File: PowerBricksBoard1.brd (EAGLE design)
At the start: 76.2 x 50.8 mm, 16 parts

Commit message: trim
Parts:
- R5: value 475k -> 510k
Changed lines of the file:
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@@
 <attribute name="VALUE" x="58.0644" y="26.3398" size="0.6096" layer="27" font="vector" ratio="20" rot="R270" align="top-center"/>
 </element>
-<element name="R5" library="SparkFun-Resistors" library_urn="urn:adsk.eagle:library:532" package="0603" package3d_urn="urn:adsk.eagle:package:39650/1" value="475k" x="60.96" y="22.733" smashed="yes" rot="R270">
+<element name="R5" library="SparkFun-Resistors" library_urn="urn:adsk.eagle:library:532" package="0603" package3d_urn="urn:adsk.eagle:package:39650/1" value="510k" x="60.96" y="22.733" smashed="yes" rot="R270">
 <attribute name="NAME" x="61.721996875" y="22.733003125" size="0.6096" layer="25" font="vector" ratio="20" rot="R270" align="bottom-center"/>
 <attribute name="PROD_ID" value=" " x="-30.479996875" y="-64.896996875" size="1.778" layer="27" rot="R270" display="off"/>

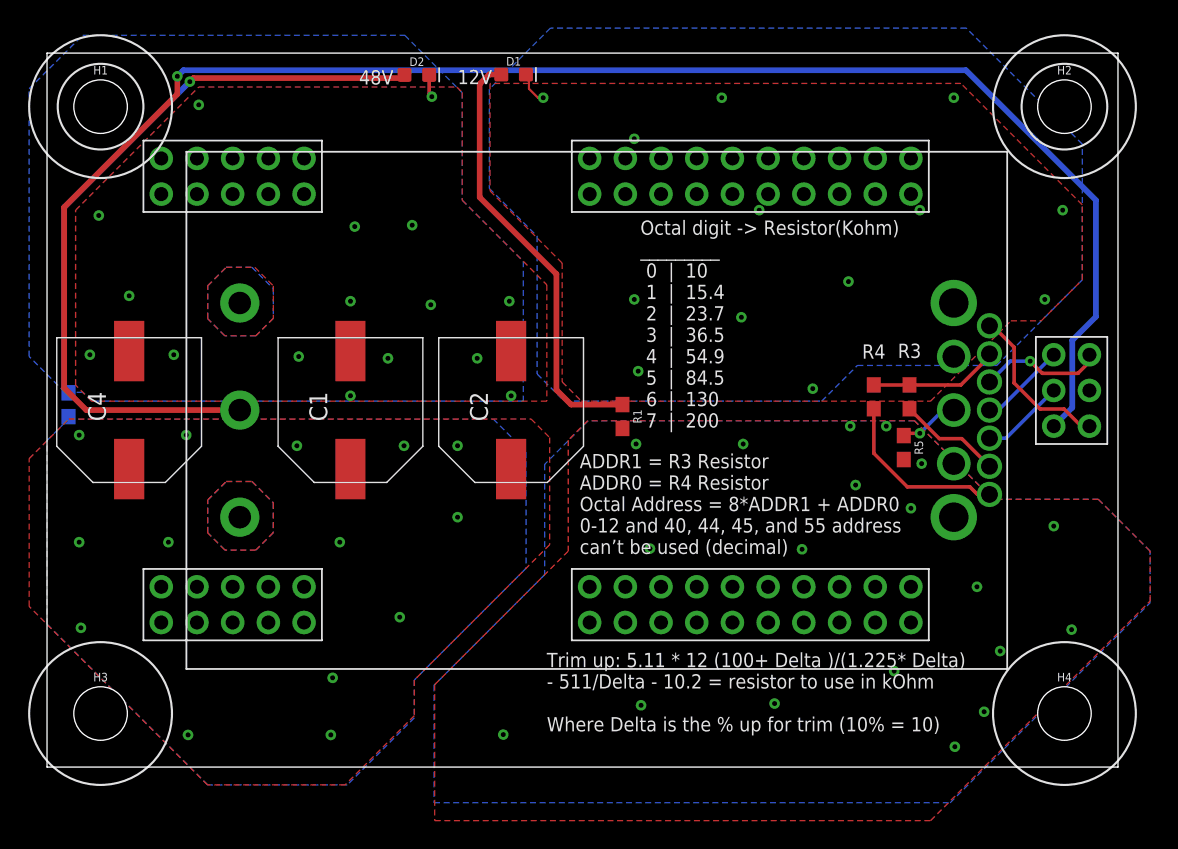
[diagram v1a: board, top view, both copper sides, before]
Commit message: Cleaning up git and exports for order
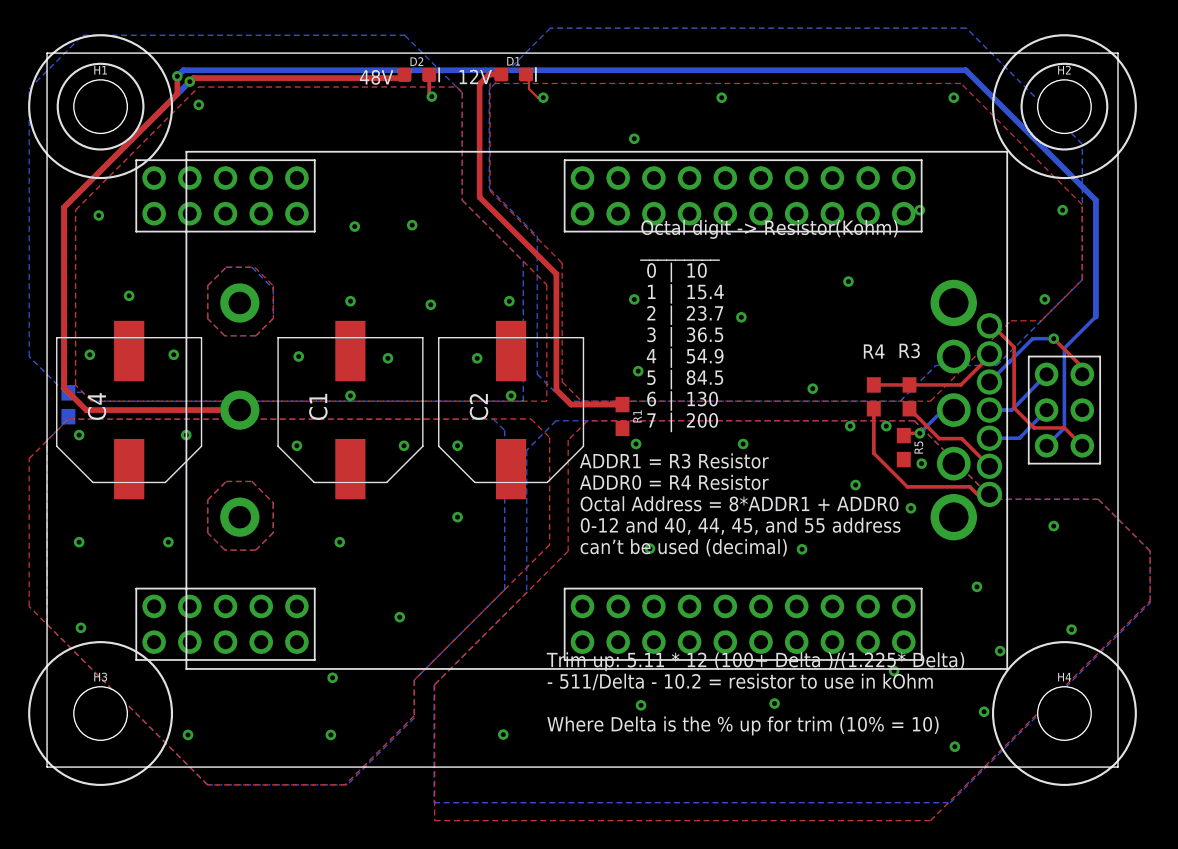
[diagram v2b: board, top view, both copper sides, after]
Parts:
- moved U$1 1.49 mm to (38.1, 25.4)
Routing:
- net ON/OFF: track 125.3 -> 126.9 mm
- net C2: track 11.6 -> 12.7 mm
- net ALERT: track 6.20 -> 5.14 mm
- net CLK: track 5.98 -> 4.92 mm
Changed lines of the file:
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@@
 <setting verticaltext="up"/>
 </settings>
-<grid distance="50" unitdist="mil" unit="mil" style="lines" multiple="1" display="no" altdistance="2" altunitdist="mil" altunit="mil"/>
+<grid distance="10" unitdist="mil" unit="mil" style="lines" multiple="1" display="no" altdistance="5" altunitdist="mil" altunit="mil"/>
 <layers>
 <layer number="1" name="Top" color="4" fill="1" visible="yes" active="yes"/>
@@
 </element>
 <element name="U$2" library="Delta Power Bricks - Q48SC12050NRDH" package="Q48SC12050NRDH" package3d_urn="urn:adsk.eagle:package:24241038/2" value="Q48SC12050NRDH" x="13.716" y="17.78" smashed="yes"/>
-<element name="U$1" library="Brick_Dist_Connector" package="BRICK2DIST_D2" value="BRICK2DIST" x="38.608" y="26.797" smashed="yes"/>
+<element name="U$1" library="Brick_Dist_Connector" package="BRICK2DIST_D2" value="BRICK2DIST" x="38.1" y="25.4" smashed="yes"/>
 </elements>
 <signals>
@@
 <vertex x="1.524" y="24.765"/>
 <vertex x="31.75" y="24.765"/>
-<vertex x="34.0868" y="22.4282"/>
-<vertex x="34.0868" y="14.1478"/>
+<vertex x="32.5628" y="23.9522"/>
+<vertex x="32.5628" y="12.6238"/>
 <vertex x="26.1366" y="6.1976"/>
 <vertex x="26.1366" y="3.5052"/>
@@
 <contactref element="U$2" pad="9"/>
 <polygon width="0.9144" layer="16" isolate="0.508">
-<vertex x="35.4076" y="13.6906"/>
+<vertex x="34.1376" y="12.4206"/>
 <vertex x="27.5336" y="5.8166"/>
 <vertex x="27.5336" y="-2.54"/>
@@
 <vertex x="67.31" y="19.05"/>
 <vertex x="61.722" y="24.638"/>
-<vertex x="38.5064" y="24.638"/>
-<vertex x="35.4076" y="21.5392"/>
+<vertex x="36.2204" y="24.638"/>
+<vertex x="34.1376" y="22.5552"/>
 </polygon>
 <polygon width="0.9144" layer="1" isolate="0.508">
@@
 <contactref element="U$2" pad="10"/>
 <contactref element="U$1" pad="A"/>
-<wire x1="74.168" y1="24.257" x2="73.5838" y2="24.257" width="0.254" layer="1"/>
-<wire x1="72.3646" y1="25.4762" x2="70.6628" y2="25.4762" width="0.254" layer="1"/>
-<wire x1="70.6628" y1="25.4762" x2="68.8086" y2="27.3304" width="0.254" layer="1"/>
-<wire x1="68.8086" y1="27.3304" x2="68.8086" y2="29.8704" width="0.254" layer="1"/>
+<wire x1="68.8086" y1="29.8704" x2="68.8086" y2="25.5524" width="0.254" layer="1"/>
 <wire x1="68.8086" y1="29.8704" x2="67.279" y2="31.4" width="0.254" layer="1"/>
 <wire x1="67.279" y1="31.4" x2="67.056" y2="31.4" width="0.254" layer="1"/>
-<wire x1="73.5838" y1="24.257" x2="72.3646" y2="25.4762" width="0.254" layer="1"/>
+<wire x1="72.39" y1="24.13" x2="73.66" y2="22.86" width="0.254" layer="1"/>
+<wire x1="68.8086" y1="25.5524" x2="70.231" y2="24.13" width="0.254" layer="1"/>
+<wire x1="70.231" y1="24.13" x2="72.39" y2="24.13" width="0.254" layer="1"/>
 </signal>
 <signal name="12_GND">
@@
 <vertex x="34.8742" y="27.9654"/>
 <vertex x="36.8046" y="26.035"/>
-<vertex x="55.118" y="26.035"/>
-<vertex x="57.658" y="28.575"/>
+<vertex x="60.706" y="26.035"/>
+<vertex x="63.246" y="28.575"/>
 <vertex x="67.564" y="28.575"/>
 <vertex x="73.66" y="34.671"/>
@@
 <wire x1="34.29" y1="48.26" x2="34.925" y2="47.625" width="0.1524" layer="1"/>
 <wire x1="34.925" y1="47.625" x2="35.306" y2="47.625" width="0.1524" layer="1"/>
+<wire x1="60.96" y1="39.37" x2="62.103" y2="39.624" width="0" layer="19" extent="1-1"/>
+<wire x1="50.673" y1="39.624" x2="50.8" y2="39.37" width="0" layer="19" extent="1-1"/>
 </signal>
 <signal name="ALERT">
 <contactref element="U$2" pad="13"/>
 <contactref element="U$1" pad="D"/>
-<wire x1="71.628" y1="29.337" x2="67.691" y2="25.4" width="0.254" layer="16"/>
-<wire x1="67.691" y1="25.4" x2="67.056" y2="25.4" width="0.254" layer="16"/>
+<wire x1="71.12" y1="27.94" x2="68.6562" y2="25.4" width="0.254" layer="16"/>
+<wire x1="68.6562" y1="25.4" x2="67.056" y2="25.4" width="0.254" layer="16"/>
 </signal>
 <signal name="DATA">
 <contactref element="U$2" pad="12"/>
 <contactref element="U$1" pad="E"/>
-<wire x1="67.056" y1="27.4" x2="68.5358" y2="28.8798" width="0.254" layer="16"/>
-<wire x1="69.9488" y1="28.8798" x2="68.5358" y2="28.8798" width="0.254" layer="16"/>
-<via x="69.9488" y="28.8798" extent="1-16" drill="0.35"/>
-<wire x1="69.9488" y1="28.8798" x2="70.8124" y2="28.0162" width="0.254" layer="1"/>
-<wire x1="70.8124" y1="28.0162" x2="73.3552" y2="28.0162" width="0.254" layer="1"/>
-<wire x1="73.3552" y1="28.0162" x2="74.168" y2="28.829" width="0.254" layer="1"/>
-<wire x1="74.168" y1="28.829" x2="74.168" y2="29.337" width="0.254" layer="1"/>
+<wire x1="67.056" y1="27.4" x2="68.469" y2="28.813" width="0.254" layer="16"/>
+<wire x1="68.469" y1="28.813" x2="68.5358" y2="28.8798" width="0.254" layer="16"/>
+<wire x1="68.5358" y1="28.8798" x2="70.136" y2="30.48" width="0.254" layer="16"/>
+<wire x1="70.136" y1="30.48" x2="71.628" y2="30.48" width="0.254" layer="16"/>
+<via x="71.628" y="30.48" extent="1-16" drill="0.35"/>
+<wire x1="71.628" y1="30.48" x2="73.66" y2="28.448" width="0.254" layer="1"/>
+<wire x1="73.66" y1="28.448" x2="73.66" y2="27.94" width="0.254" layer="1"/>
 </signal>
 <signal name="CLK">
 <contactref element="U$2" pad="14"/>
 <contactref element="U$1" pad="C"/>
-<wire x1="71.628" y1="26.797" x2="68.231" y2="23.4" width="0.254" layer="16"/>
-<wire x1="68.231" y1="23.4" x2="67.056" y2="23.4" width="0.254" layer="16"/>
+<wire x1="71.12" y1="25.4" x2="69.1962" y2="23.4" width="0.254" layer="16"/>
+<wire x1="69.1962" y1="23.4" x2="67.056" y2="23.4" width="0.254" layer="16"/>
 </signal>
 <signal name="N$1">
@@
 <wire x1="65.3809125" y1="49.5808" x2="74.62585625" y2="40.33585625" width="0.4064" layer="16"/>
 <contactref element="U$1" pad="B"/>
-<wire x1="74.62585625" y1="40.33585625" x2="74.62585625" y2="32.04195" width="0.4064" layer="16"/>
-<wire x1="72.9488" y1="25.5778" x2="71.628" y2="24.257" width="0.4064" layer="16"/>
-<wire x1="74.62585625" y1="32.04195" x2="72.9488" y2="30.36489375" width="0.4064" layer="16"/>
-<wire x1="72.9488" y1="30.36489375" x2="72.9488" y2="25.5778" width="0.4064" layer="16"/>
+<wire x1="74.62585625" y1="32.04195" x2="74.62585625" y2="40.33585625" width="0.4064" layer="16"/>
+<wire x1="71.12" y1="22.86" x2="72.39" y2="24.13" width="0.254" layer="16"/>
+<wire x1="72.39" y1="29.80609375" x2="74.62585625" y2="32.04195" width="0.254" layer="16"/>
+<wire x1="72.39" y1="24.13" x2="72.39" y2="29.80609375" width="0.254" layer="16"/>
 </signal>
 </signals>
